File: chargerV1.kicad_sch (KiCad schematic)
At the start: 47 parts, among them J1 USB_C_Receptacle, J2 SOCKET_1x4, J3 SOCKET_1x4, J4 SOCKET_1x6, J5 Micro_SD_Card, SW1 BOOT, SW2 OK, SW3 RESET, SW4 UP, SW5 DW, U1 DS3231M, U2 ESP32-WROOM-32D, U4 AMS1117-3.3

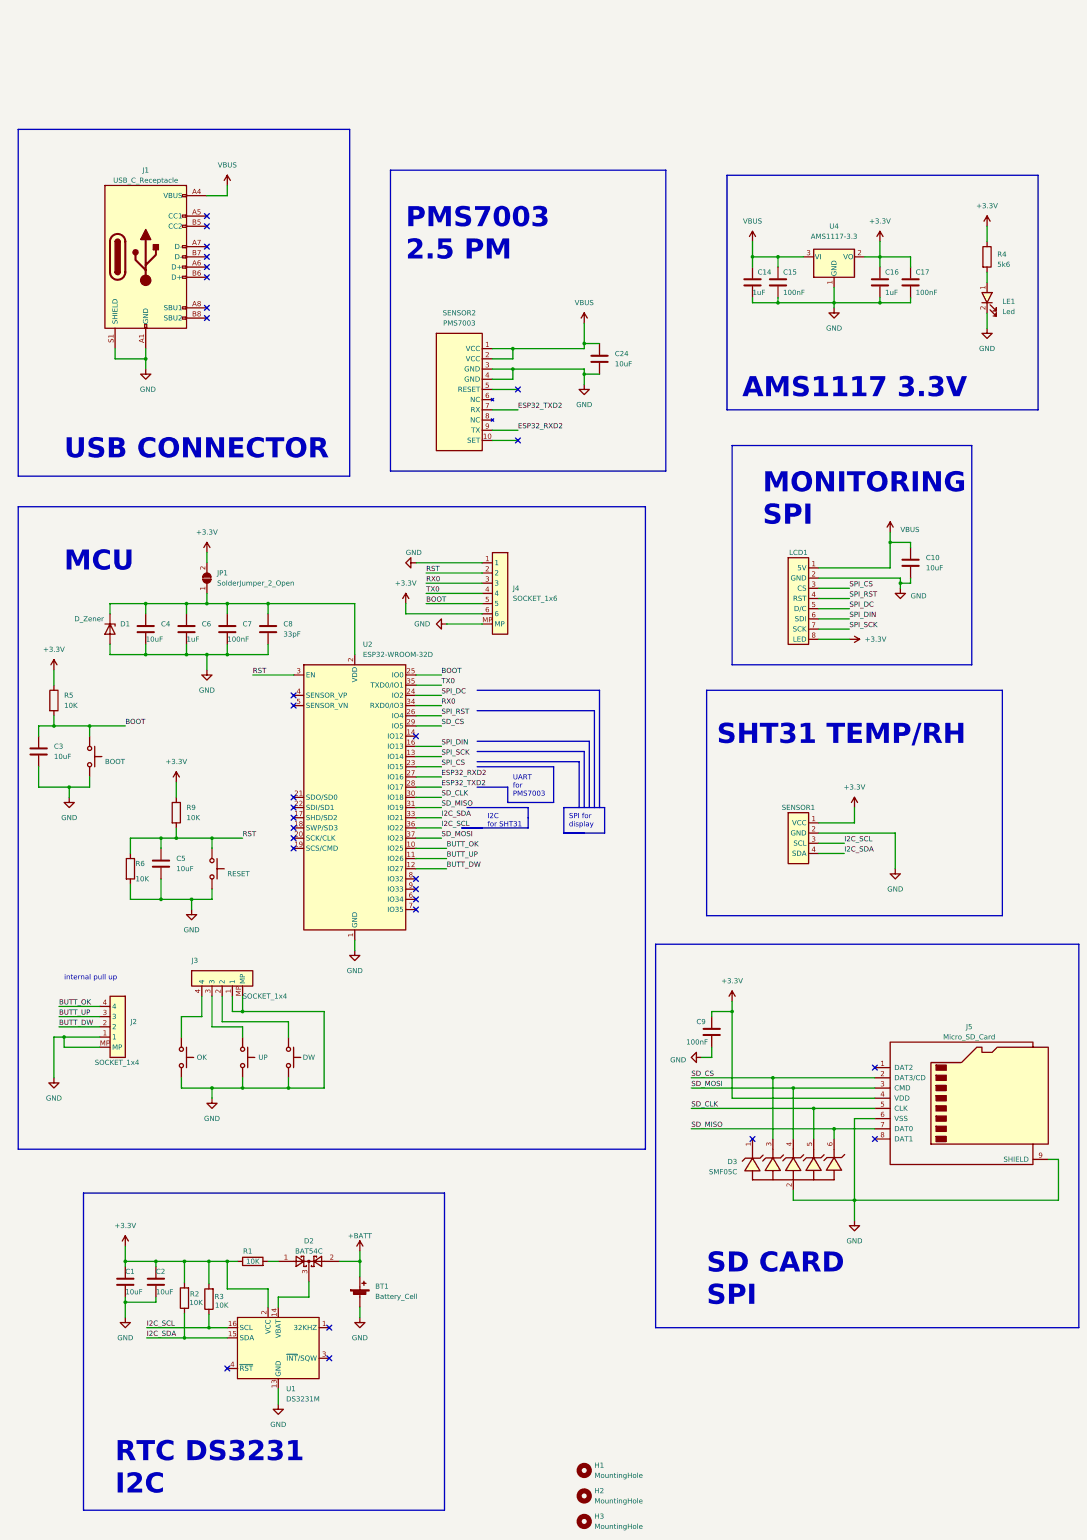
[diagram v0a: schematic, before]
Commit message: Fix buttons
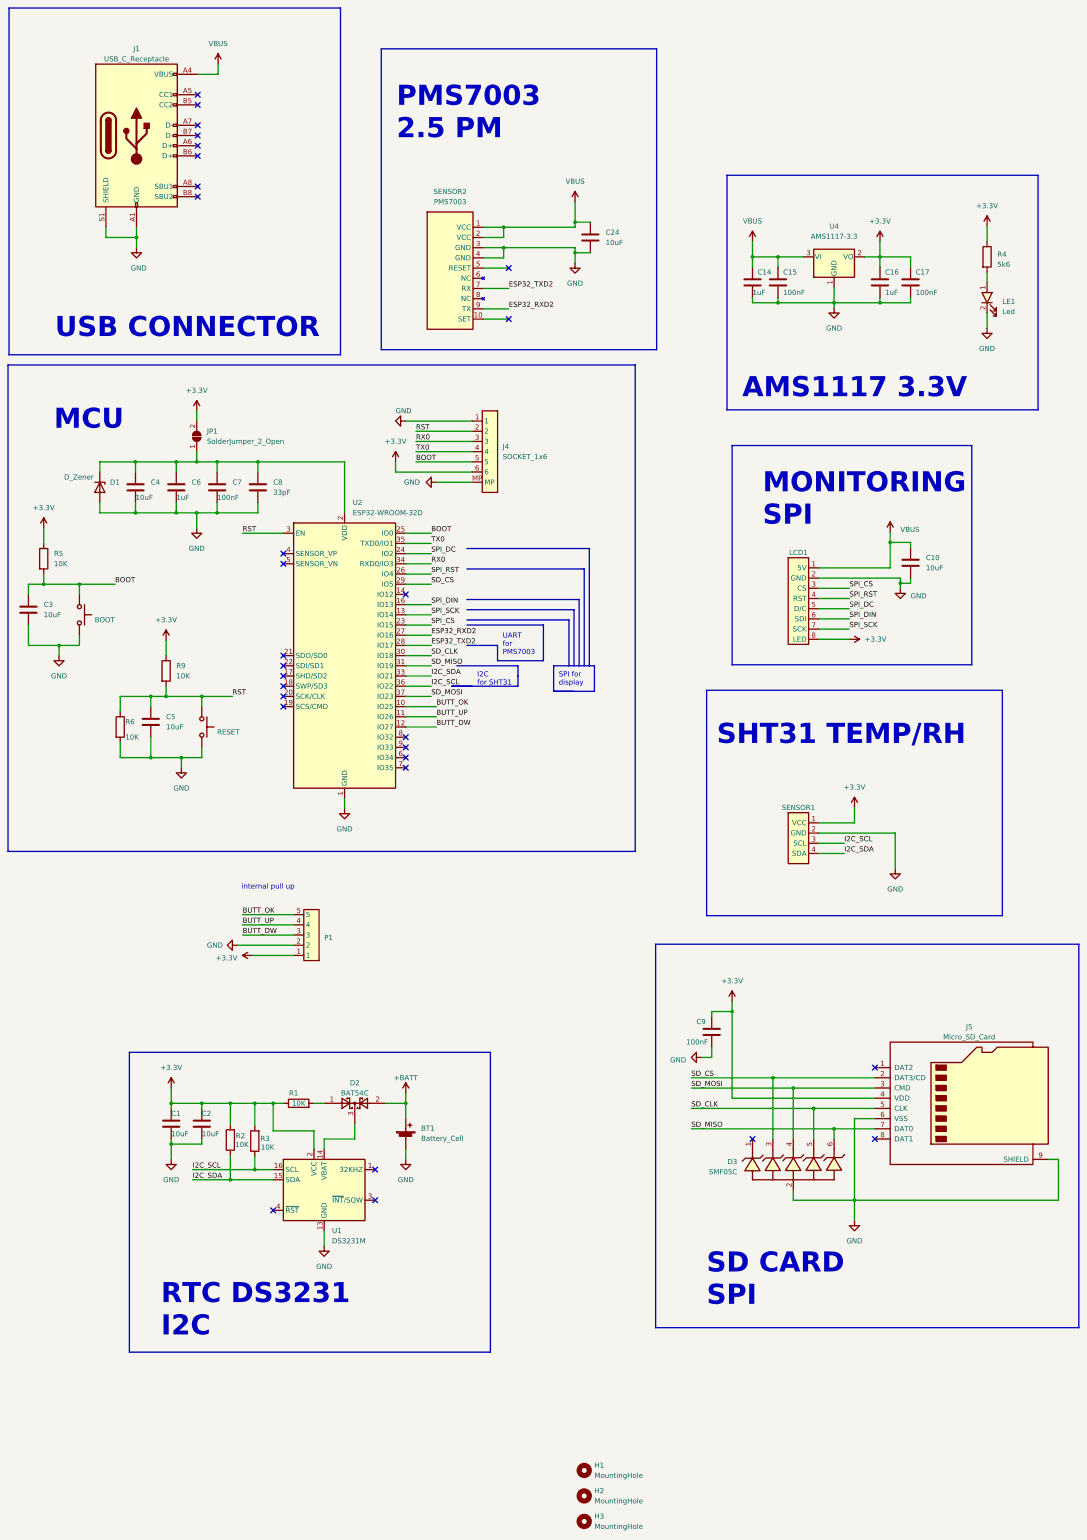
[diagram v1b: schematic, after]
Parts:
- removed J2, J3: SOCKET_1x4, IVS_footprints:JST_SH_SM04B-SRSS-TB_1x04-1MP_P1.00mm_Horizontal, symbol IVS_symbol:SOCKET_1x4
- removed SW2: OK, IVS_footprints:Button_Push_12mm, symbol IVS_SYMBOL:switch
- removed SW4: UP, IVS_footprints:Button_Push_12mm, symbol IVS_SYMBOL:switch
- removed SW5: DW, IVS_footprints:Button_Push_12mm, symbol IVS_SYMBOL:switch
- added P1: ~, IVS_footprints:JST_SH_SM05B-SRSS-TB_1x05-1MP_P1.00mm_Horizontal, symbol IVS_symbols:SOCKET_1x5
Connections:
- net +3.3V: now also P1.1
- net BUTT_DW: now also P1.3
- net BUTT_OK: now also P1.5
- net BUTT_UP: now also P1.4
- net GND: now also P1.2
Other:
- moved on the sheet: BT1, C1, C2, C24, C3, C4, C5, C6, C7, C8, D1, D2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
